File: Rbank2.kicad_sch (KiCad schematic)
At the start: 100 parts, among them K24 TQ2-5, K25 TQ2-5, K26 TQ2-5, K27 TQ2-5, K28 TQ2-5, K29 TQ2-5, K30 TQ2-5, K31 TQ2-5, K32 TQ2-5, Q40 2N2222, Q41 2N2222, Q42 2N2222, Q43 2N2222, Q44 2N2222, Q45 2N2222, Q46 2N2222, Q47 2N2222, Q48 2N2222

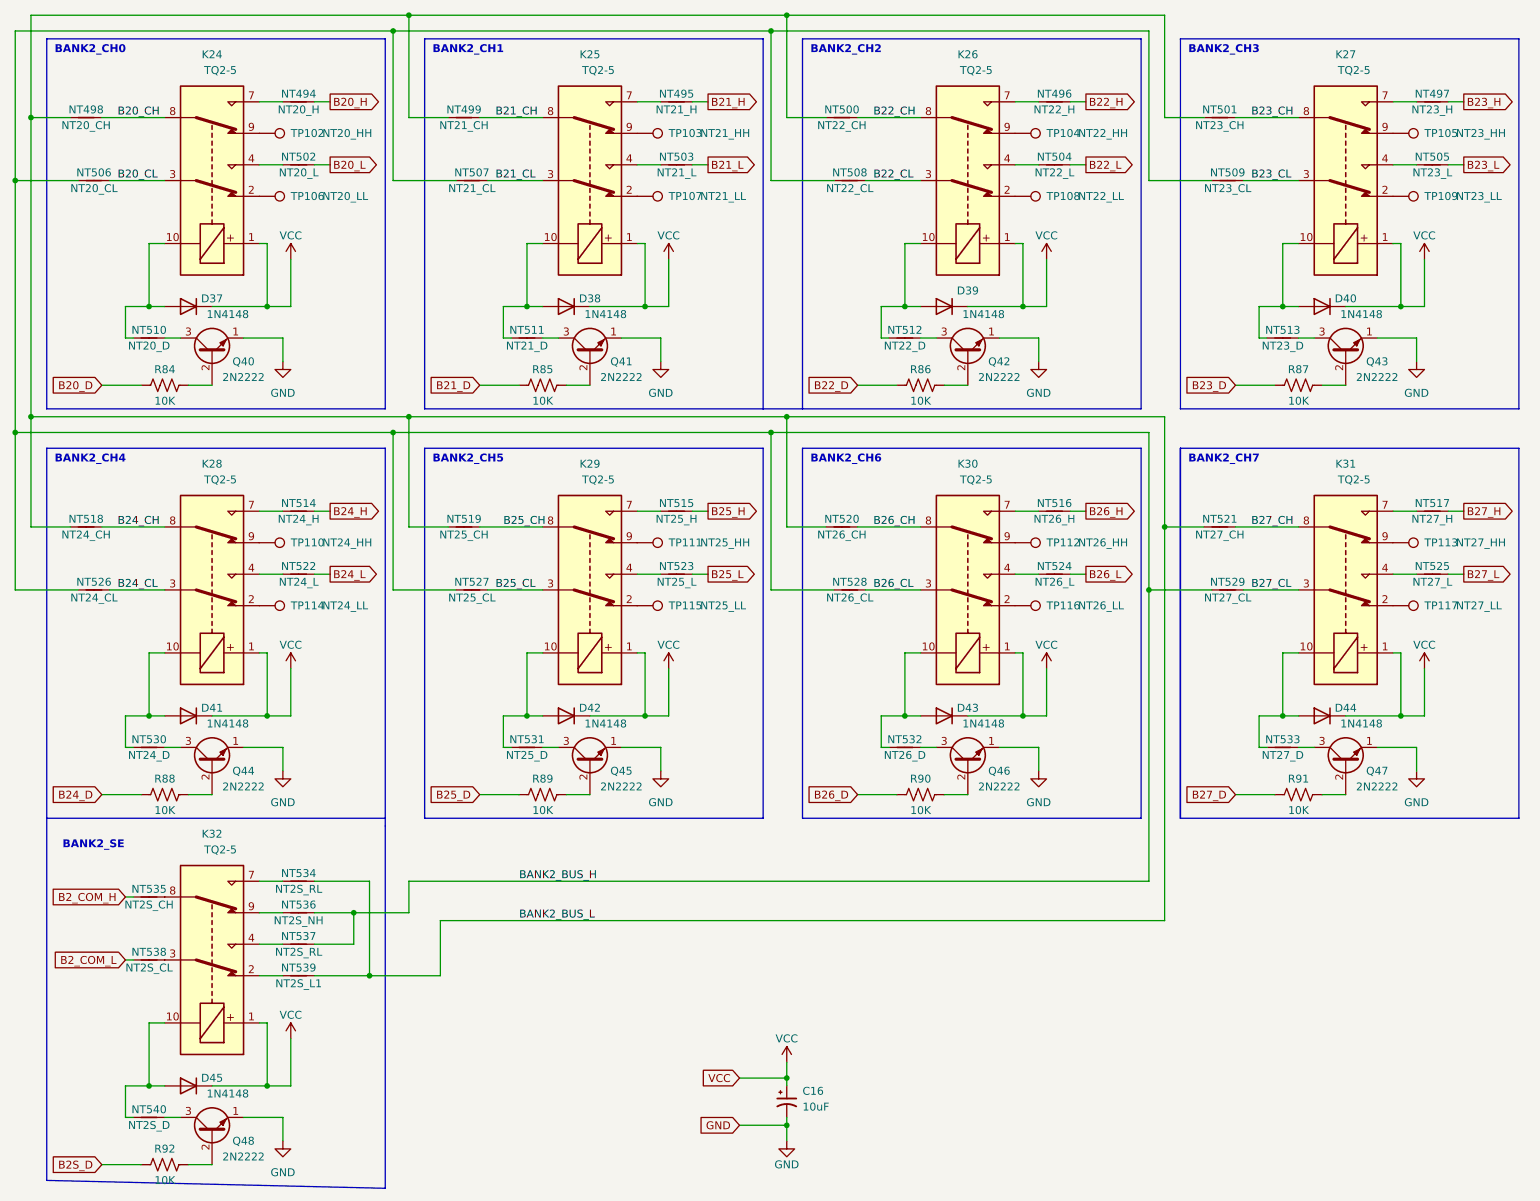
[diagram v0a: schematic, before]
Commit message: backup 1 bank done
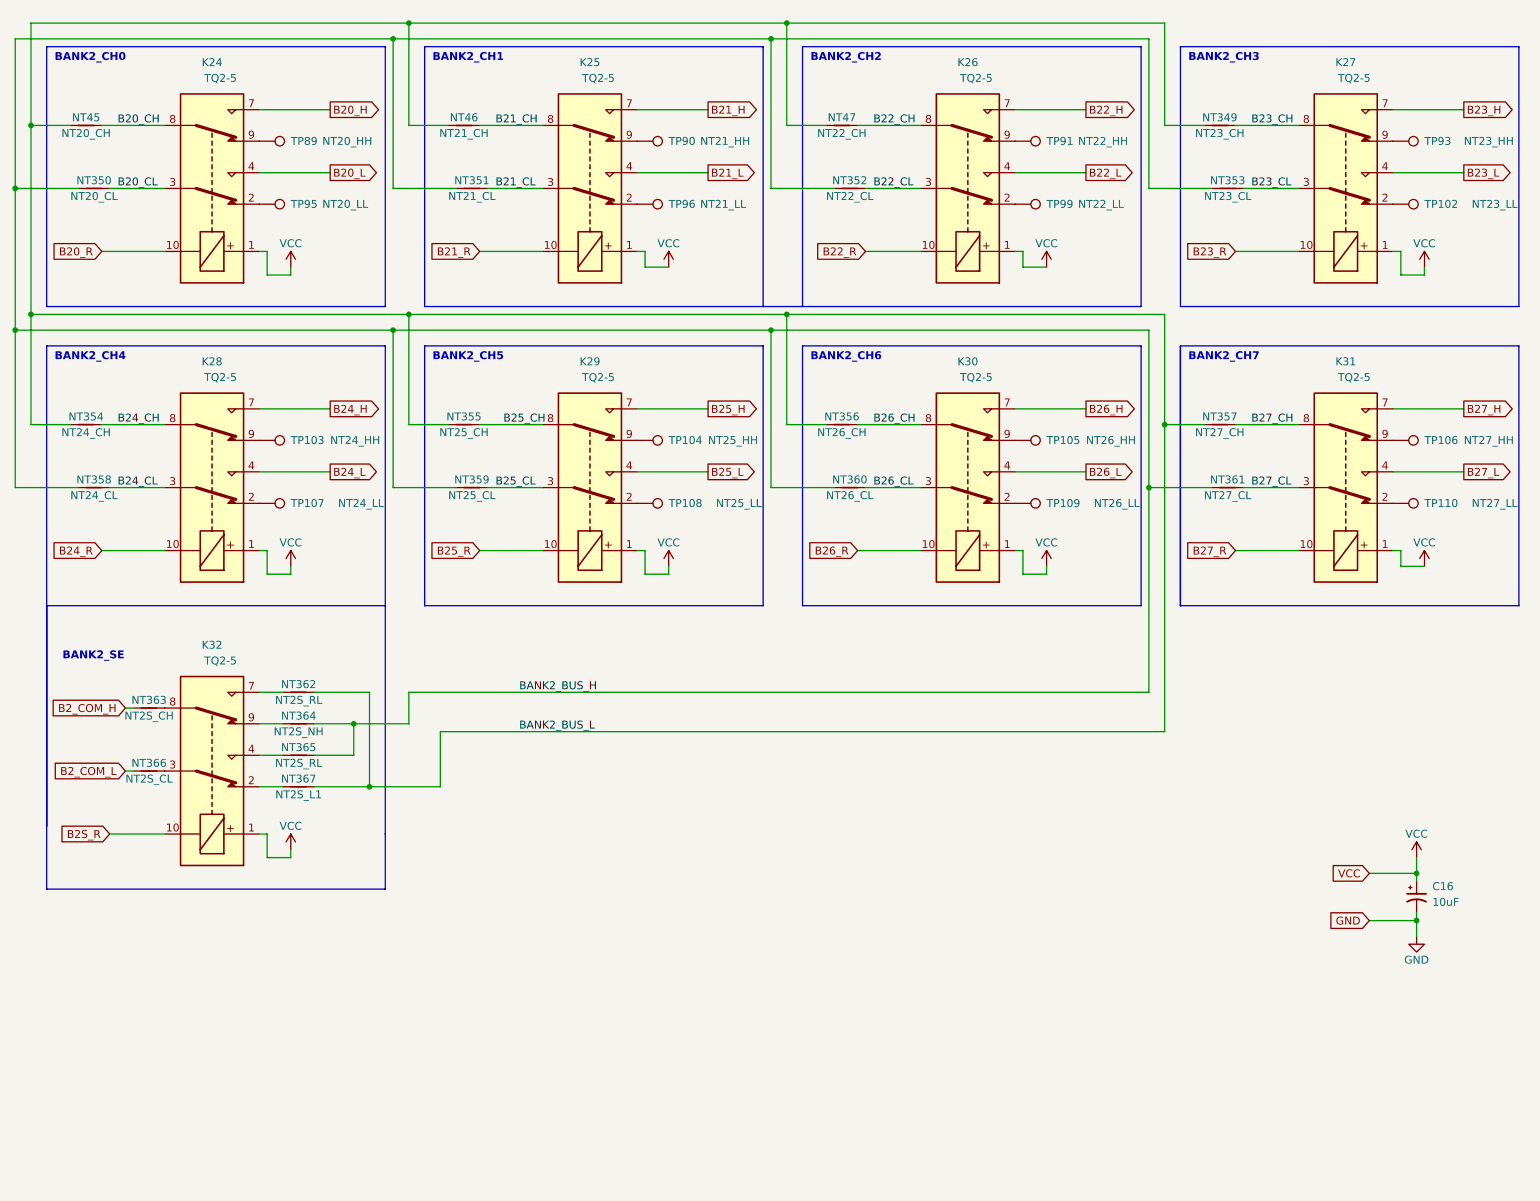
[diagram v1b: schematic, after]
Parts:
- removed D37, D38, D39, D40, D41, D42, D43, D44, D45: 1N4148, Diode_THT:D_DO-35_SOD27_P7.62mm_Horizontal, symbol Diode:1N4148
- removed NT494: NT20_H, NetTie:NetTie-2_THT_Pad1.0mm, symbol Device:NetTie_2
- removed NT495: NT21_H, NetTie:NetTie-2_THT_Pad1.0mm, symbol Device:NetTie_2
- removed NT496: NT22_H, NetTie:NetTie-2_THT_Pad1.0mm, symbol Device:NetTie_2
- removed NT497: NT23_H, NetTie:NetTie-2_THT_Pad1.0mm, symbol Device:NetTie_2
- removed NT498: NT20_CH, NetTie:NetTie-2_THT_Pad1.0mm, symbol Device:NetTie_2
- removed NT499: NT21_CH, NetTie:NetTie-2_THT_Pad1.0mm, symbol Device:NetTie_2
- removed NT500: NT22_CH, NetTie:NetTie-2_THT_Pad1.0mm, symbol Device:NetTie_2
- removed NT501: NT23_CH, NetTie:NetTie-2_THT_Pad1.0mm, symbol Device:NetTie_2
- removed NT502: NT20_L, NetTie:NetTie-2_THT_Pad1.0mm, symbol Device:NetTie_2
- removed NT503: NT21_L, NetTie:NetTie-2_THT_Pad1.0mm, symbol Device:NetTie_2
- removed NT504: NT22_L, NetTie:NetTie-2_THT_Pad1.0mm, symbol Device:NetTie_2
- removed NT505: NT23_L, NetTie:NetTie-2_THT_Pad1.0mm, symbol Device:NetTie_2
- removed NT506: NT20_CL, NetTie:NetTie-2_THT_Pad1.0mm, symbol Device:NetTie_2
- removed NT507: NT21_CL, NetTie:NetTie-2_THT_Pad1.0mm, symbol Device:NetTie_2
- removed NT508: NT22_CL, NetTie:NetTie-2_THT_Pad1.0mm, symbol Device:NetTie_2
- removed NT509: NT23_CL, NetTie:NetTie-2_THT_Pad1.0mm, symbol Device:NetTie_2
- removed NT510: NT20_D, NetTie:NetTie-2_THT_Pad1.0mm, symbol Device:NetTie_2
- removed NT511: NT21_D, NetTie:NetTie-2_THT_Pad1.0mm, symbol Device:NetTie_2
- removed NT512: NT22_D, NetTie:NetTie-2_THT_Pad1.0mm, symbol Device:NetTie_2
- removed NT513: NT23_D, NetTie:NetTie-2_THT_Pad1.0mm, symbol Device:NetTie_2
- removed NT514: NT24_H, NetTie:NetTie-2_THT_Pad1.0mm, symbol Device:NetTie_2
- removed NT515: NT25_H, NetTie:NetTie-2_THT_Pad1.0mm, symbol Device:NetTie_2
- removed NT516: NT26_H, NetTie:NetTie-2_THT_Pad1.0mm, symbol Device:NetTie_2
- removed NT517: NT27_H, NetTie:NetTie-2_THT_Pad1.0mm, symbol Device:NetTie_2
- removed NT518: NT24_CH, NetTie:NetTie-2_THT_Pad1.0mm, symbol Device:NetTie_2
- removed NT519: NT25_CH, NetTie:NetTie-2_THT_Pad1.0mm, symbol Device:NetTie_2
- removed NT520: NT26_CH, NetTie:NetTie-2_THT_Pad1.0mm, symbol Device:NetTie_2
- removed NT521: NT27_CH, NetTie:NetTie-2_THT_Pad1.0mm, symbol Device:NetTie_2
- removed NT522: NT24_L, NetTie:NetTie-2_THT_Pad1.0mm, symbol Device:NetTie_2
- removed NT523: NT25_L, NetTie:NetTie-2_THT_Pad1.0mm, symbol Device:NetTie_2
- removed NT524: NT26_L, NetTie:NetTie-2_THT_Pad1.0mm, symbol Device:NetTie_2
- removed NT525: NT27_L, NetTie:NetTie-2_THT_Pad1.0mm, symbol Device:NetTie_2
- removed NT526: NT24_CL, NetTie:NetTie-2_THT_Pad1.0mm, symbol Device:NetTie_2
- removed NT527: NT25_CL, NetTie:NetTie-2_THT_Pad1.0mm, symbol Device:NetTie_2
- removed NT528: NT26_CL, NetTie:NetTie-2_THT_Pad1.0mm, symbol Device:NetTie_2
- removed NT529: NT27_CL, NetTie:NetTie-2_THT_Pad1.0mm, symbol Device:NetTie_2
- removed NT530: NT24_D, NetTie:NetTie-2_THT_Pad1.0mm, symbol Device:NetTie_2
- removed NT531: NT25_D, NetTie:NetTie-2_THT_Pad1.0mm, symbol Device:NetTie_2
- removed NT532: NT26_D, NetTie:NetTie-2_THT_Pad1.0mm, symbol Device:NetTie_2
- removed NT533: NT27_D, NetTie:NetTie-2_THT_Pad1.0mm, symbol Device:NetTie_2
- removed NT534, NT537: NT2S_RL, NetTie:NetTie-2_THT_Pad1.0mm, symbol Device:NetTie_2
- removed NT535: NT2S_CH, NetTie:NetTie-2_THT_Pad1.0mm, symbol Device:NetTie_2
- removed NT536: NT2S_NH, NetTie:NetTie-2_THT_Pad1.0mm, symbol Device:NetTie_2
- removed NT538: NT2S_CL, NetTie:NetTie-2_THT_Pad1.0mm, symbol Device:NetTie_2
- removed NT539: NT2S_L1, NetTie:NetTie-2_THT_Pad1.0mm, symbol Device:NetTie_2
- removed NT540: NT2S_D, NetTie:NetTie-2_THT_Pad1.0mm, symbol Device:NetTie_2
- removed Q40, Q41, Q42, Q43, Q44, Q45, Q46, Q47, Q48: 2N2222, Package_TO_SOT_THT:TO-92_Inline, symbol Transistor_BJT:2N3904
- removed R84, R85, R86, R87, R88, R89, R90, R91, R92: 10K, Resistor_THT:R_Axial_DIN0309_L9.0mm_D3.2mm_P12.70mm_Horizontal, symbol Device:R_US
- removed TP111: NT25_HH, Connector_Pin:Pin_D1.0mm_L10.0mm, symbol Connector:TestPoint
- removed TP112: NT26_HH, Connector_Pin:Pin_D1.0mm_L10.0mm, symbol Connector:TestPoint
- removed TP113: NT27_HH, Connector_Pin:Pin_D1.0mm_L10.0mm, symbol Connector:TestPoint
- removed TP114: NT24_LL, Connector_Pin:Pin_D1.0mm_L10.0mm, symbol Connector:TestPoint
- removed TP115: NT25_LL, Connector_Pin:Pin_D1.0mm_L10.0mm, symbol Connector:TestPoint
- removed TP116: NT26_LL, Connector_Pin:Pin_D1.0mm_L10.0mm, symbol Connector:TestPoint
- removed TP117: NT27_LL, Connector_Pin:Pin_D1.0mm_L10.0mm, symbol Connector:TestPoint
- added NT349: NT23_CH, NetTie:NetTie-2_Front1.0mm, symbol Device:NetTie_2
- added NT350: NT20_CL, NetTie:NetTie-2_Front1.0mm, symbol Device:NetTie_2
- added NT351: NT21_CL, NetTie:NetTie-2_Front1.0mm, symbol Device:NetTie_2
- added NT352: NT22_CL, NetTie:NetTie-2_Front1.0mm, symbol Device:NetTie_2
- added NT353: NT23_CL, NetTie:NetTie-2_Front1.0mm, symbol Device:NetTie_2
- added NT354: NT24_CH, NetTie:NetTie-2_Front1.0mm, symbol Device:NetTie_2
- added NT355: NT25_CH, NetTie:NetTie-2_Front1.0mm, symbol Device:NetTie_2
- added NT356: NT26_CH, NetTie:NetTie-2_Front1.0mm, symbol Device:NetTie_2
- added NT357: NT27_CH, NetTie:NetTie-2_Front1.0mm, symbol Device:NetTie_2
- added NT358: NT24_CL, NetTie:NetTie-2_Front1.0mm, symbol Device:NetTie_2
- added NT359: NT25_CL, NetTie:NetTie-2_Front1.0mm, symbol Device:NetTie_2
- added NT360: NT26_CL, NetTie:NetTie-2_Front1.0mm, symbol Device:NetTie_2
- added NT361: NT27_CL, NetTie:NetTie-2_Front1.0mm, symbol Device:NetTie_2
- added NT362, NT365: NT2S_RL, NetTie:NetTie-2_Front1.0mm, symbol Device:NetTie_2
- added NT363: NT2S_CH, NetTie:NetTie-2_Front1.0mm, symbol Device:NetTie_2
- added NT364: NT2S_NH, NetTie:NetTie-2_Front1.0mm, symbol Device:NetTie_2
- added NT366: NT2S_CL, NetTie:NetTie-2_Front1.0mm, symbol Device:NetTie_2
- added NT367: NT2S_L1, NetTie:NetTie-2_Front1.0mm, symbol Device:NetTie_2
- added NT45: NT20_CH, NetTie:NetTie-2_Front1.0mm, symbol Device:NetTie_2
- added NT46: NT21_CH, NetTie:NetTie-2_Front1.0mm, symbol Device:NetTie_2
- added NT47: NT22_CH, NetTie:NetTie-2_Front1.0mm, symbol Device:NetTie_2
- added TP89: NT20_HH, Connector_Pin:Pin_D0.9mm_L10.0mm_W2.4mm_FlatFork, symbol Connector:TestPoint
- added TP90: NT21_HH, Connector_Pin:Pin_D0.9mm_L10.0mm_W2.4mm_FlatFork, symbol Connector:TestPoint
- added TP91: NT22_HH, Connector_Pin:Pin_D0.9mm_L10.0mm_W2.4mm_FlatFork, symbol Connector:TestPoint
- added TP93: NT23_HH, Connector_Pin:Pin_D0.9mm_L10.0mm_W2.4mm_FlatFork, symbol Connector:TestPoint
- added TP95: NT20_LL, Connector_Pin:Pin_D0.9mm_L10.0mm_W2.4mm_FlatFork, symbol Connector:TestPoint
- added TP96: NT21_LL, Connector_Pin:Pin_D0.9mm_L10.0mm_W2.4mm_FlatFork, symbol Connector:TestPoint
- added TP99: NT22_LL, Connector_Pin:Pin_D0.9mm_L10.0mm_W2.4mm_FlatFork, symbol Connector:TestPoint
- TP102: value NT20_HH -> NT23_LL; footprint Connector_Pin:Pin_D1.0mm_L10.0mm -> Connector_Pin:Pin_D0.9mm_L10.0mm_W2.4mm_FlatFork
- TP103: value NT21_HH -> NT24_HH; footprint Connector_Pin:Pin_D1.0mm_L10.0mm -> Connector_Pin:Pin_D0.9mm_L10.0mm_W2.4mm_FlatFork
- TP104: value NT22_HH -> NT25_HH; footprint Connector_Pin:Pin_D1.0mm_L10.0mm -> Connector_Pin:Pin_D0.9mm_L10.0mm_W2.4mm_FlatFork
- TP105: value NT23_HH -> NT26_HH; footprint Connector_Pin:Pin_D1.0mm_L10.0mm -> Connector_Pin:Pin_D0.9mm_L10.0mm_W2.4mm_FlatFork
- TP106: value NT20_LL -> NT27_HH; footprint Connector_Pin:Pin_D1.0mm_L10.0mm -> Connector_Pin:Pin_D0.9mm_L10.0mm_W2.4mm_FlatFork
- TP107: value NT21_LL -> NT24_LL; footprint Connector_Pin:Pin_D1.0mm_L10.0mm -> Connector_Pin:Pin_D0.9mm_L10.0mm_W2.4mm_FlatFork
- TP108: value NT22_LL -> NT25_LL; footprint Connector_Pin:Pin_D1.0mm_L10.0mm -> Connector_Pin:Pin_D0.9mm_L10.0mm_W2.4mm_FlatFork
- TP109: value NT23_LL -> NT26_LL; footprint Connector_Pin:Pin_D1.0mm_L10.0mm -> Connector_Pin:Pin_D0.9mm_L10.0mm_W2.4mm_FlatFork
- TP110: value NT24_HH -> NT27_LL; footprint Connector_Pin:Pin_D1.0mm_L10.0mm -> Connector_Pin:Pin_D0.9mm_L10.0mm_W2.4mm_FlatFork
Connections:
- net B20_CH: now also NT45.2
- net B20_CL: now also NT350.2
- net B20_H: now also K24.7
- net B20_L: now also K24.4
- net B21_CH: now also NT46.2
- net B21_CL: now also NT351.2
- net B21_H: now also K25.7
- net B21_L: now also K25.4
- net B22_CH: now also NT47.2
- net B22_CL: now also NT352.2
- net B22_H: now also K26.7
- net B22_L: now also K26.4
- net B23_CH: now also NT349.2
- net B23_CL: now also NT353.2
- net B23_H: now also K27.7
- net B23_L: now also K27.4
- net B24_CH: now also NT354.2
- net B24_CL: now also NT358.2
- net B24_H: now also K28.7
- net B24_L: now also K28.4
- net B25_CH: now also NT355.2
- net B25_CL: now also NT359.2
- net B25_H: now also K29.7
- net B25_L: now also K29.4
- net B26_CH: now also NT356.2
- net B26_CL: now also NT360.2
- net B26_H: now also K30.7
- net B26_L: now also K30.4
- net B27_CH: now also NT357.2
- net B27_CL: now also NT361.2
- net B27_H: now also K31.7
- net B27_L: now also K31.4
- net B2_COM_H: now also NT363.1
- net B2_COM_L: now also NT366.1
- net BANK2_BUS_H: now also NT350.1, NT351.1, NT352.1, NT353.1, NT358.1, NT359.1, NT360.1, NT361.1, NT364.2, NT365.2
- net BANK2_BUS_L: now also NT349.1, NT354.1, NT355.1, NT356.1, NT357.1, NT362.2, NT367.2, NT45.1, NT46.1, NT47.1
- net B23_R: now reaches K27.10
- net at TP109.1: now also K30.2; no longer K27.2
- net at TP105.1: now also K30.9; no longer K27.9
- net B21_R: now reaches K25.10
- net at K26.2: now also TP99.1; no longer TP108.1
- net B25_R: now reaches K29.10
- net B2S_R: now reaches K32.10
- net at K28.9: now also TP103.1; no longer TP110.1
- net at K25.9: now also TP90.1; no longer TP103.1
- net at K26.9: now also TP91.1; no longer TP104.1
- net at K31.2: now also TP110.1
- net at K32.2: now also NT367.1
- net at K32.3: now also NT366.2
- net at K32.4: now also NT365.1
- net at K32.7: now also NT362.1
- net at K32.8: now also NT363.2
- net at K32.9: now also NT364.1
- net B20_R: now reaches K24.10
- net at K24.2: now also TP95.1; no longer TP106.1
- net B26_R: now reaches K30.10
- net B27_R: now reaches K31.10
- net at TP107.1: now also K28.2; no longer K25.2
- net at K24.9: now also TP89.1; no longer TP102.1
- net B22_R: now reaches K26.10
- net at K29.9: now also TP104.1
- net B24_R: now reaches K28.10
- net at K29.2: now also TP108.1
- net at K31.9: now also TP106.1
- new net: K27.2, TP102.1
- new net: K27.9, TP93.1
- new net: K25.2, TP96.1

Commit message: PCB Completed
PCB completed but final verification not completed
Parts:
- TP102, TP103, TP104, TP105, TP106, TP107, TP108, TP109, TP110, TP89, TP90, TP91, TP93, TP95, TP96, TP99: footprint Connector_Pin:Pin_D0.9mm_L10.0mm_W2.4mm_FlatFork -> TestPoint:TestPoint_THTPad_D1.5mm_Drill0.7mm
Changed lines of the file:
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@@
       (effects (font (size 1.27 1.27)) (justify left))
     )
-    (property "Footprint" "Connector_Pin:Pin_D0.9mm_L10.0mm_W2.4mm_FlatFork" (id 2) (at 54.61 87.63 0)
+    (property "Footprint" "TestPoint:TestPoint_THTPad_D1.5mm_Drill0.7mm" (id 2) (at 54.61 87.63 0)
       (effects (font (size 1.27 1.27)) hide)
     )
@@
       (effects (font (size 1.27 1.27)) (justify left))
     )
-    (property "Footprint" "Connector_Pin:Pin_D0.9mm_L10.0mm_W2.4mm_FlatFork" (id 2) (at 176.53 49.53 0)
+    (property "Footprint" "TestPoint:TestPoint_THTPad_D1.5mm_Drill0.7mm" (id 2) (at 176.53 49.53 0)
       (effects (font (size 1.27 1.27)) hide)
     )
@@
       (effects (font (size 1.27 1.27)) (justify left))
     )
-    (property "Footprint" "Connector_Pin:Pin_D0.9mm_L10.0mm_W2.4mm_FlatFork" (id 2) (at 237.49 97.79 0)
+    (property "Footprint" "TestPoint:TestPoint_THTPad_D1.5mm_Drill0.7mm" (id 2) (at 237.49 97.79 0)
       (effects (font (size 1.27 1.27)) hide)
     )
@@
       (effects (font (size 1.27 1.27)) (justify left))
     )
-    (property "Footprint" "Connector_Pin:Pin_D0.9mm_L10.0mm_W2.4mm_FlatFork" (id 2) (at 115.57 97.79 0)
+    (property "Footprint" "TestPoint:TestPoint_THTPad_D1.5mm_Drill0.7mm" (id 2) (at 115.57 97.79 0)
       (effects (font (size 1.27 1.27)) hide)
     )
@@
       (effects (font (size 1.27 1.27)) (justify left))
     )
-    (property "Footprint" "Connector_Pin:Pin_D0.9mm_L10.0mm_W2.4mm_FlatFork" (id 2) (at 176.53 87.63 0)
+    (property "Footprint" "TestPoint:TestPoint_THTPad_D1.5mm_Drill0.7mm" (id 2) (at 176.53 87.63 0)
       (effects (font (size 1.27 1.27)) hide)
     )
@@
       (effects (font (size 1.27 1.27)) (justify left))
     )
-    (property "Footprint" "Connector_Pin:Pin_D0.9mm_L10.0mm_W2.4mm_FlatFork" (id 2) (at 176.53 97.79 0)
+    (property "Footprint" "TestPoint:TestPoint_THTPad_D1.5mm_Drill0.7mm" (id 2) (at 176.53 97.79 0)
       (effects (font (size 1.27 1.27)) hide)
     )
@@
       (effects (font (size 1.27 1.27)) (justify left))
     )
-    (property "Footprint" "Connector_Pin:Pin_D0.9mm_L10.0mm_W2.4mm_FlatFork" (id 2) (at 54.61 49.53 0)
+    (property "Footprint" "TestPoint:TestPoint_THTPad_D1.5mm_Drill0.7mm" (id 2) (at 54.61 49.53 0)
       (effects (font (size 1.27 1.27)) hide)
     )
@@
       (effects (font (size 1.27 1.27)) (justify left))
     )
-    (property "Footprint" "Connector_Pin:Pin_D0.9mm_L10.0mm_W2.4mm_FlatFork" (id 2) (at 237.49 49.53 0)
+    (property "Footprint" "TestPoint:TestPoint_THTPad_D1.5mm_Drill0.7mm" (id 2) (at 237.49 49.53 0)
       (effects (font (size 1.27 1.27)) hide)
     )
@@
       (effects (font (size 1.27 1.27)) (justify left))
     )
-    (property "Footprint" "Connector_Pin:Pin_D0.9mm_L10.0mm_W2.4mm_FlatFork" (id 2) (at 54.61 39.37 0)
+    (property "Footprint" "TestPoint:TestPoint_THTPad_D1.5mm_Drill0.7mm" (id 2) (at 54.61 39.37 0)
       (effects (font (size 1.27 1.27)) hide)
     )
@@
       (effects (font (size 1.27 1.27)) (justify left))
     )
-    (property "Footprint" "Connector_Pin:Pin_D0.9mm_L10.0mm_W2.4mm_FlatFork" (id 2) (at 115.57 87.63 0)
+    (property "Footprint" "TestPoint:TestPoint_THTPad_D1.5mm_Drill0.7mm" (id 2) (at 115.57 87.63 0)
       (effects (font (size 1.27 1.27)) hide)
     )
@@
       (effects (font (size 1.27 1.27)) (justify left))
     )
-    (property "Footprint" "Connector_Pin:Pin_D0.9mm_L10.0mm_W2.4mm_FlatFork" (id 2) (at 237.49 87.63 0)
+    (property "Footprint" "TestPoint:TestPoint_THTPad_D1.5mm_Drill0.7mm" (id 2) (at 237.49 87.63 0)
       (effects (font (size 1.27 1.27)) hide)
     )
@@
       (effects (font (size 1.27 1.27)) (justify left))
     )
-    (property "Footprint" "Connector_Pin:Pin_D0.9mm_L10.0mm_W2.4mm_FlatFork" (id 2) (at 237.49 39.37 0)
+    (property "Footprint" "TestPoint:TestPoint_THTPad_D1.5mm_Drill0.7mm" (id 2) (at 237.49 39.37 0)
       (effects (font (size 1.27 1.27)) hide)
     )
@@
       (effects (font (size 1.27 1.27)) (justify left))
     )
-    (property "Footprint" "Connector_Pin:Pin_D0.9mm_L10.0mm_W2.4mm_FlatFork" (id 2) (at 115.57 39.37 0)
+    (property "Footprint" "TestPoint:TestPoint_THTPad_D1.5mm_Drill0.7mm" (id 2) (at 115.57 39.37 0)
       (effects (font (size 1.27 1.27)) hide)
     )
@@
       (effects (font (size 1.27 1.27)) (justify left))
     )
-    (property "Footprint" "Connector_Pin:Pin_D0.9mm_L10.0mm_W2.4mm_FlatFork" (id 2) (at 54.61 97.79 0)
+    (property "Footprint" "TestPoint:TestPoint_THTPad_D1.5mm_Drill0.7mm" (id 2) (at 54.61 97.79 0)
       (effects (font (size 1.27 1.27)) hide)
     )
@@
       (effects (font (size 1.27 1.27)) (justify left))
     )
-    (property "Footprint" "Connector_Pin:Pin_D0.9mm_L10.0mm_W2.4mm_FlatFork" (id 2) (at 115.57 49.53 0)
+    (property "Footprint" "TestPoint:TestPoint_THTPad_D1.5mm_Drill0.7mm" (id 2) (at 115.57 49.53 0)
       (effects (font (size 1.27 1.27)) hide)
     )
@@
       (effects (font (size 1.27 1.27)) (justify left))
     )
-    (property "Footprint" "Connector_Pin:Pin_D0.9mm_L10.0mm_W2.4mm_FlatFork" (id 2) (at 176.53 39.37 0)
-      (effects (font (size 1.27 1.27)) hide)
-    )
+    (property "Footprint" "TestPoint:TestPoint_THTPad_D1.5mm_Drill0.7mm" (id 2) (at 176.53 39.37 0)
+      (effects (font (size 1.27 1.27)) hide)
+    )
